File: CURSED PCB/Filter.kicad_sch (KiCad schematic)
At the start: 5 parts, among them U8 LT6023

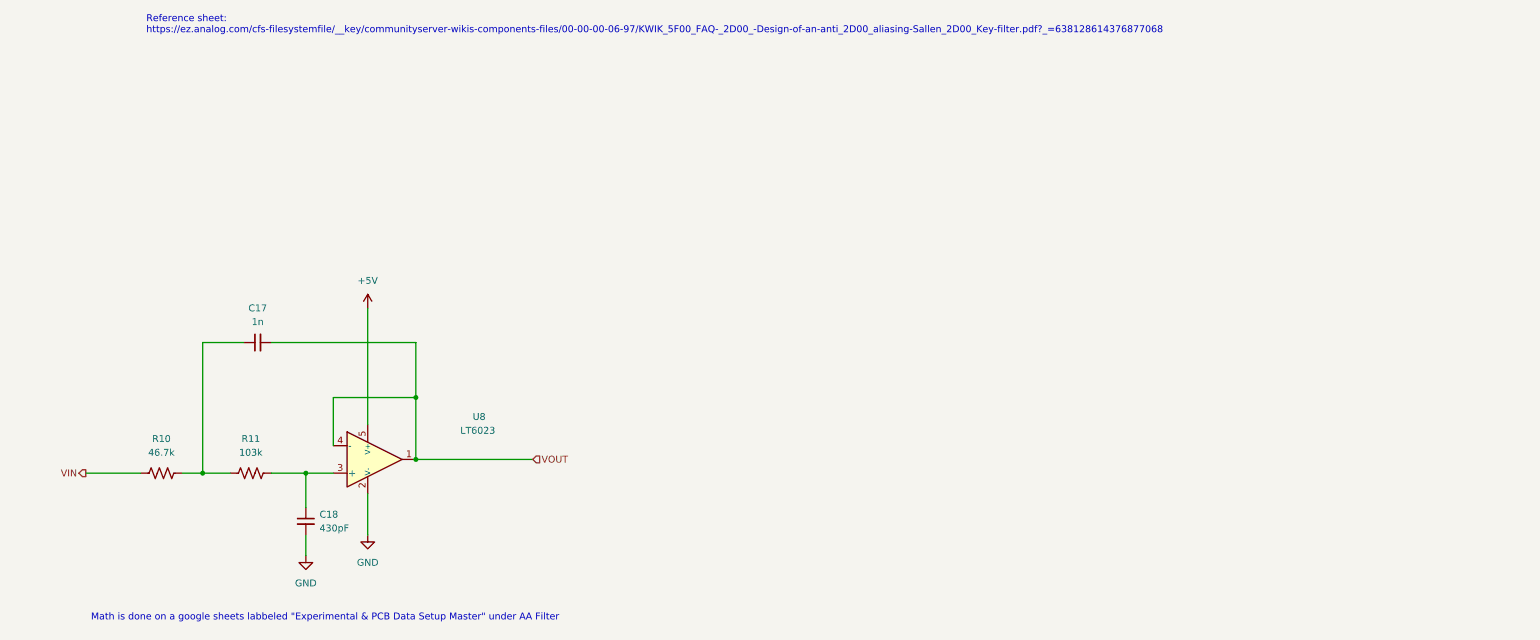
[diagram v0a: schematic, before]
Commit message: text for reviwers
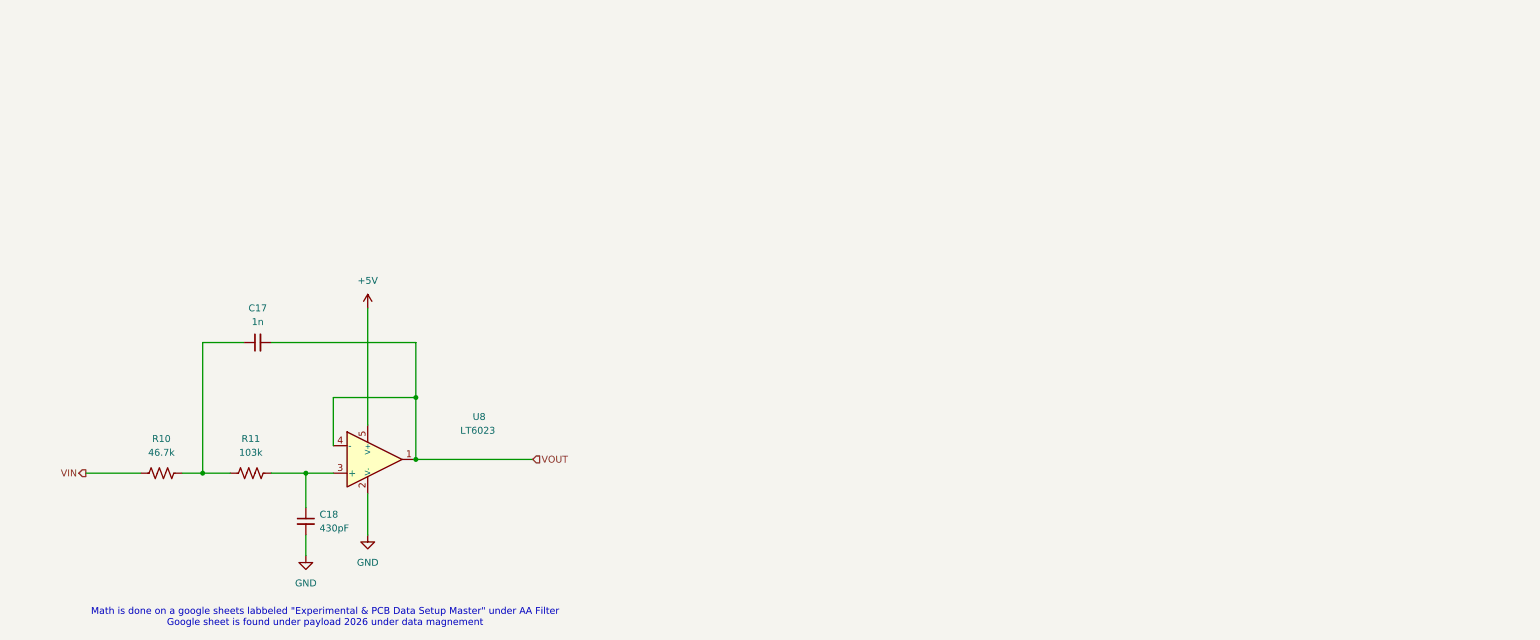
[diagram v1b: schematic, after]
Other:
- note added: "Math is done on a google sheets labbeled "Experimental & PCB Data Setup Master" under AA Filter Google sheet is found under payload 2026 under data magnement"
- note removed: "Math is done on a google sheets labbeled "Experimental & PCB Data Setup Master" under AA Filter"
- note removed: "Reference sheet: https://ez.analog.com/cfs-filesystemfile/__key/communityserver-wikis-components-files/00-00-00-06-97/KWIK_5F00_FAQ-_2D00_-Design-of-an-anti_2D00_aliasing-Sallen_2D00_Key-filter.pdf?_=638128614376877068"
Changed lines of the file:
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@@
 	(generator_version "9.0")
 	(paper "A4")
-	(text "Math is done on a google sheets labbeled \"Experimental & PCB Data Setup Master\" under AA Filter\n"
+	(text "Math is done on a google sheets labbeled \"Experimental & PCB Data Setup Master\" under AA Filter\nGoogle sheet is found under payload 2026 under data magnement "
 		(exclude_from_sim no)
 		(at 94.996 127 0)
@@
 		)
 	)
-	(text "Reference sheet:\nhttps://ez.analog.com/cfs-filesystemfile/__key/communityserver-wikis-components-files/00-00-00-06-97/KWIK_5F00_FAQ-_2D00_-Design-of-an-anti_2D00_aliasing-Sallen_2D00_Key-filter.pdf?_=638128614376877068"
-		(exclude_from_sim no)
-		(at 61.976 17.526 0)
-		(effects
-			(font
-				(size 1.27 1.27)
-			)
-			(justify left)
-		)
-	)
